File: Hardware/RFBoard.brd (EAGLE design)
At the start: 100 x 100 mm, 327 parts, among them IC1 HMC1097, IC10 NCP702-1.8, IC11 QPC6082, IC12 MCP4812, IC13 QPC6082, IC14 LT5560, IC15 ADF4360, IC16 HMC284, IC17 HMC284, IC18 NCP702-3.3, IC19 NCP702-3.3, IC2 MAX2871, IC20 LT1395, IC21 MAADSS0008, IC22 MAADSS0008, IC23 MAADSS0008, IC24 RFSA2033, IC25 MMG3H21NT1, IC26 MMG3H21NT1, IC27 HMC1021, IC28 MCP4812, IC29 NCP702-3.3, IC3 AP2114HA-3.3, IC30 NCP702-3.3, IC4 NCP702-3.3, IC5 NCP702-3.3, IC6 MAX5873, IC7 NCP702-1.8, IC8 NCP702-3.3, IC9 NCP702-3.3, Q1 BSS123, Q2 BSS123, Q3 BSS123, Q4 BSS123, Q5 BSS123, X1 out

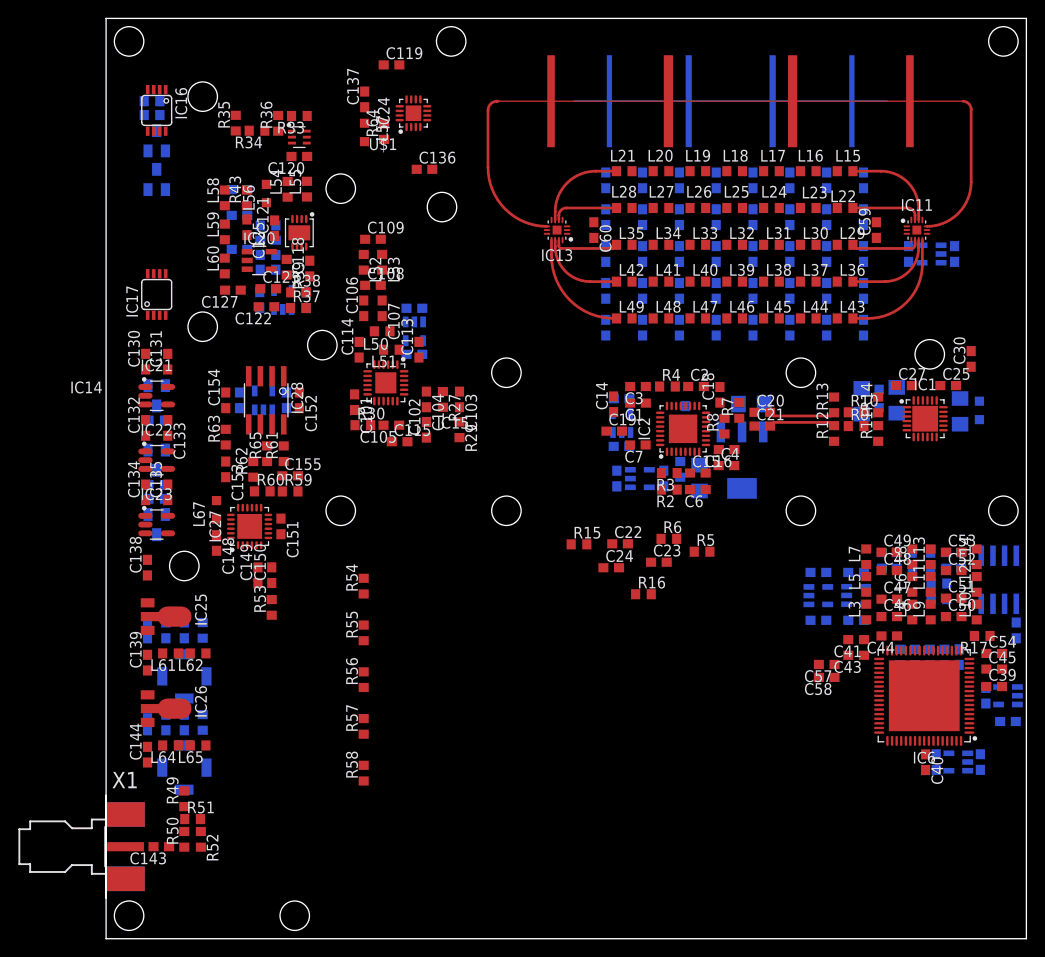
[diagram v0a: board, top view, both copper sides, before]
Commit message: Almost all RF routing
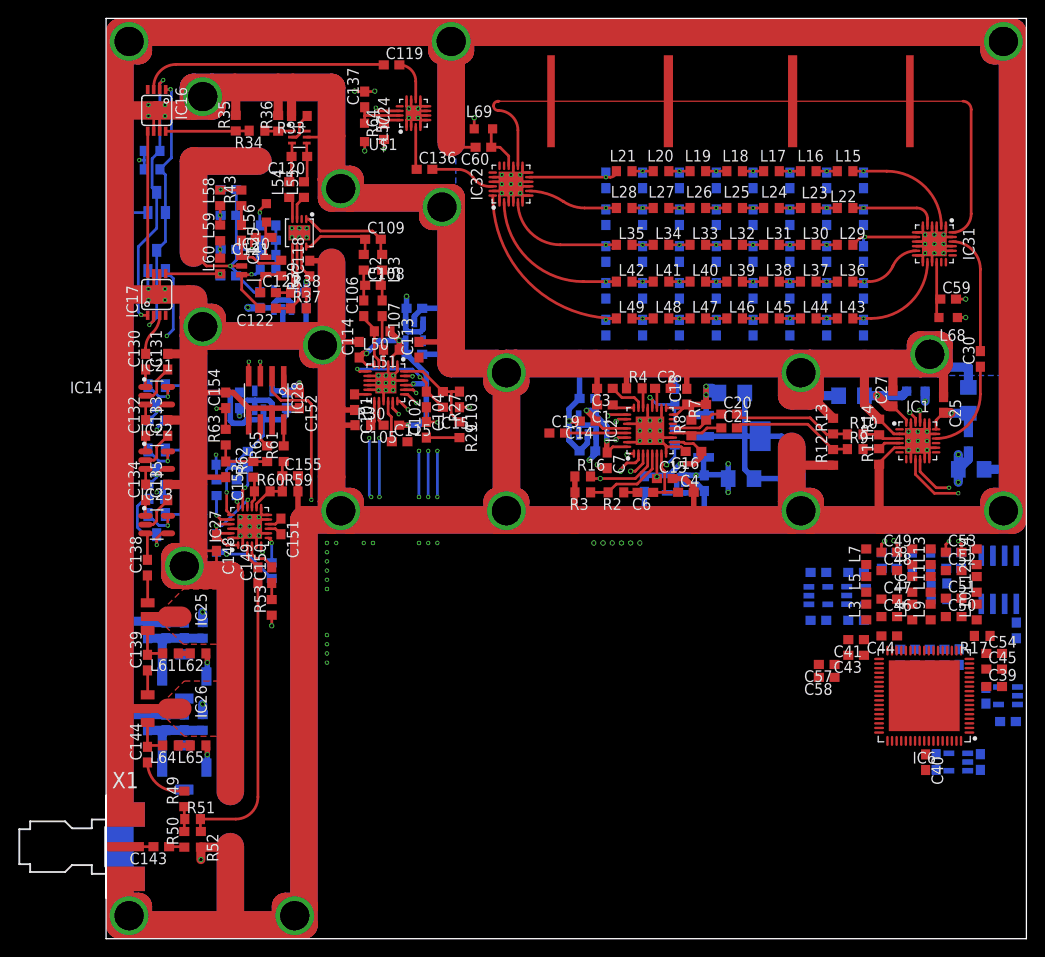
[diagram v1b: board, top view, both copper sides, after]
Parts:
- removed C157, C158: 1u, rcl:C0603
- removed C22, C23, C24: 33p, rcl:C0603
- removed IC11, IC13: QPC6082, rf:QFN40P200X200X60-15T98
- removed IC30: NCP702-3.3, rf:SOT95P240X110-5
- removed R15, R5, R6: 33, resistor:R0603
- added IC31, IC32: QPC6064, rf:QFN50P400X400X75-25T270
- added L68, L69: (no value), rcl:L2012C
- moved R58 36.4 mm to (15.4, 52.1), flipped to the bottom
- moved R57 29.4 mm to (14.2, 49.0), flipped to the bottom
- moved R56 26.3 mm to (12.0, 49.0), flipped to the bottom, turned to 270 degrees
- moved R55 23.8 mm to (12.8, 51.5), flipped to the bottom, turned to 180 degrees
- moved C60 15.0 mm to (41.0, 86.0), turned to 180 degrees
- moved R16 14.4 mm to (51.8, 50.2)
- moved C29 14.0 mm to (94.0, 51.0), turned to 180 degrees
- moved C59 10.8 mm to (91.5, 69.5), turned to 0 degrees
- moved R54 10.1 mm to (18.0, 40.0), flipped to the bottom
- moved R3 9.63 mm to (51.8, 48.5)
- moved C10 9.51 mm to (65.0, 49.5)
- moved Q1 8.80 mm to (5.50, 73.7)
- moved Q2 6.70 mm to (5.50, 80.0)
- moved C19 6.20 mm to (49.0, 55.0)
- moved R31 5.90 mm to (5.00, 83.6)
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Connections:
- removed net N$19: C22.2, IC2.1, R5.2
- removed net N$21: C24.2, IC2.3, R15.2
- removed net N$24: C23.2, IC2.2, R6.2
- removed net N$89: IC11.8, IC13.10
- removed net STEPPED37: IC11.11, IC13.7
- new net ETOUT: IC27.6
- new net VDD2: C59.1, IC31.16, L68.2
- net +5V: now also L68.1, L69.1; no longer C158.1, IC30.1, IC30.3
- net FILTERED: now also IC32.22; no longer IC13.9
- net GND: now also IC16.9, IC17.9, IC31.1, IC31.10, IC31.12, IC31.13, IC31.15, IC31.20, IC31.21, IC31.23, IC31.25, IC31.3, IC31.4, IC31.6, IC31.7, IC31.9, IC32.1, IC32.10, IC32.12, IC32.13, IC32.15, IC32.20, IC32.21, IC32.23, IC32.25, IC32.3, IC32.4, IC32.6, IC32.7, IC32.9; no longer C157.2, C158.2, C22.1, C23.1, C24.1, IC11.14, IC11.15, IC13.14, IC13.15, IC30.2
- net MOD_OUT: now also IC31.22; no longer IC11.9
- net N$52: now also IC31.2; no longer IC11.12
- net N$53: now also IC32.11; no longer IC13.6
- net N$60: now also IC31.5; no longer IC11.13
- net N$69: now also IC32.5; no longer IC13.13
- net N$76: now also IC31.11; no longer IC11.6
- net N$77: now also IC32.2; no longer IC13.12
- net N$84: now also IC31.14; no longer IC11.7
- net N$85: now also IC32.24; no longer IC13.11
- net N$90: now also IC31.8; no longer IC11.5
- net N$91: now also IC32.8; no longer IC13.5
- net SPI_CLK: now also IC2.1; no longer R5.1
- net SPI_MOSI: now also IC2.2; no longer R6.1
- net STEPPED25: now also IC31.24, IC32.14; no longer IC11.10, IC13.8
- net SW1_CTL1: now also IC31.17; no longer IC11.3
- net SW1_CTL2: now also IC31.18; no longer IC11.2
- net SW1_CTL3: now also IC31.19; no longer IC11.1
- net SW2_CTL1: now also IC32.17; no longer IC13.3
- net SW2_CTL2: now also IC32.18; no longer IC13.2
- net SW2_CTL3: now also IC32.19; no longer IC13.1
- net SWITCHES_VCC: now also IC32.16, L69.2; no longer C157.1, C59.1, IC11.4, IC13.4, IC30.5
- net SYNTH_LE: now also IC2.3; no longer R15.1
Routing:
- net GND: track 0.00 -> 1922.2 mm, vias 0 -> 102
- net +5V: track 0.00 -> 70.8 mm, vias 0 -> 21
- net EN_DIREKT: track 0.00 -> 60.9 mm, vias 0 -> 2
- net SPI_MOSI: track 0.00 -> 51.4 mm, vias 0 -> 7
- net 15DB1: track 0.00 -> 49.6 mm, vias 0 -> 2
- net SPI_CLK: track 0.00 -> 47.4 mm, vias 0 -> 7
- net GAIN_CTRL: track 0.00 -> 45.9 mm, vias 0 -> 2
- net 15DB2: track 0.00 -> 41.3 mm, vias 0 -> 2
- net N$154: track 0.00 -> 39.1 mm, vias 0 -> 4
- net STEPPED37: track 34.1 -> 0.00 mm
- net 15DB3: track 0.00 -> 32.8 mm, vias 0 -> 2
- net N$152: track 0.00 -> 31.9 mm
- net SW_HET: track 0.00 -> 29.1 mm, vias 0 -> 2
- net SW_DIRECT: track 0.00 -> 28.9 mm, vias 0 -> 2
- net PLL_DIG3: track 0.00 -> 27.2 mm, vias 0 -> 4
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- added copper zone on layer 15, net +5V
- added copper zone on layer 1, net GND
- added copper zone on layer 16, net GND
- added copper zone on layer 2, net GND
